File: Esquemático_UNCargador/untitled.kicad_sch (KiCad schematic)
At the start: 18 parts, among them U3.3 LM2596S-3.3, U5 LM2596S-5

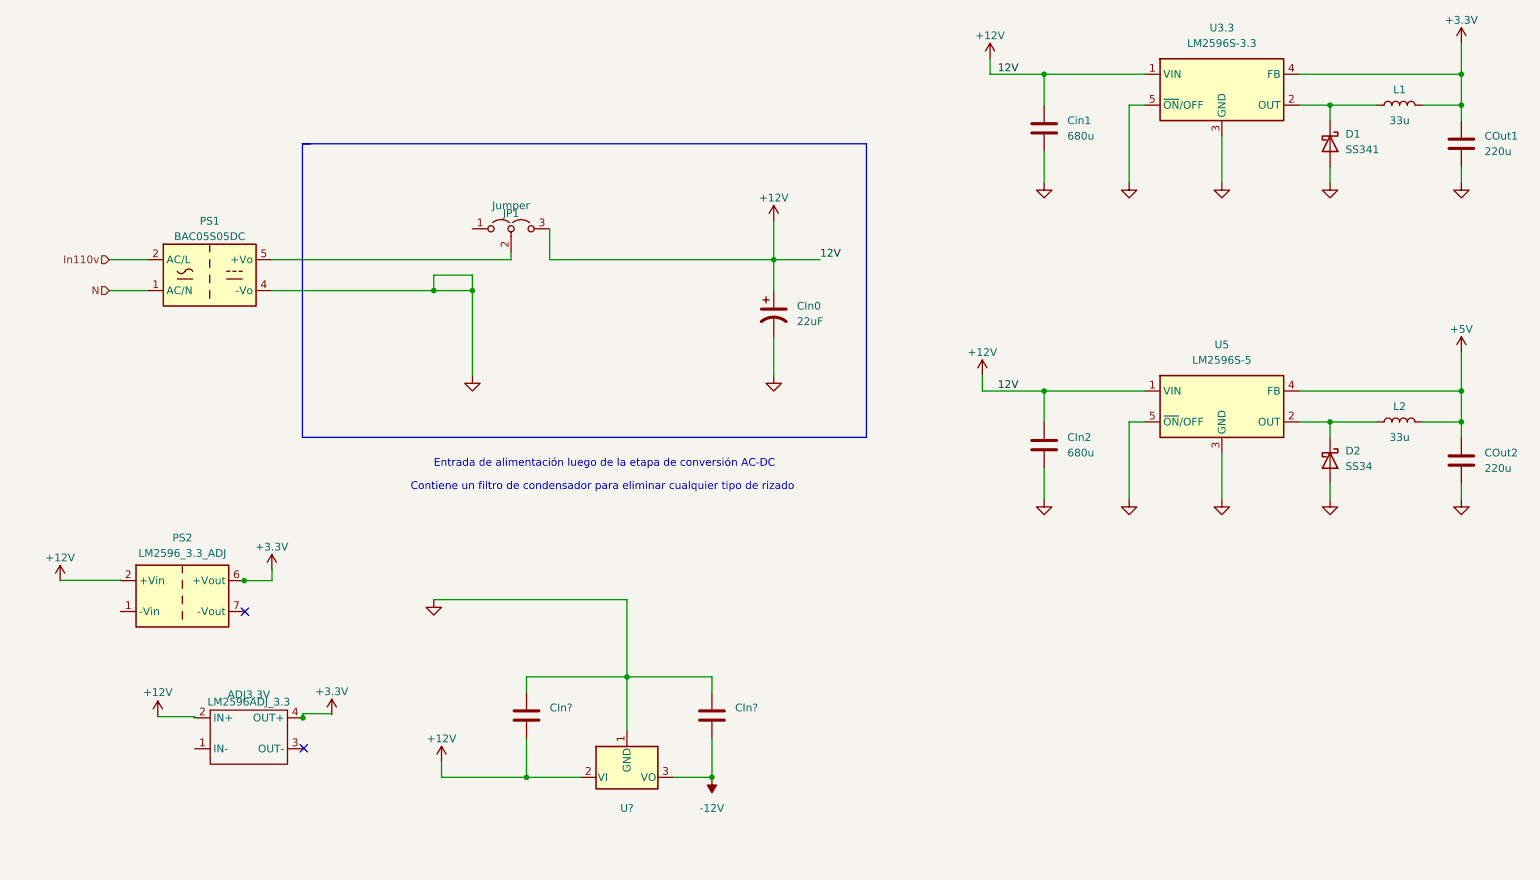
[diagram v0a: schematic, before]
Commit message: CorrecciónPotencia
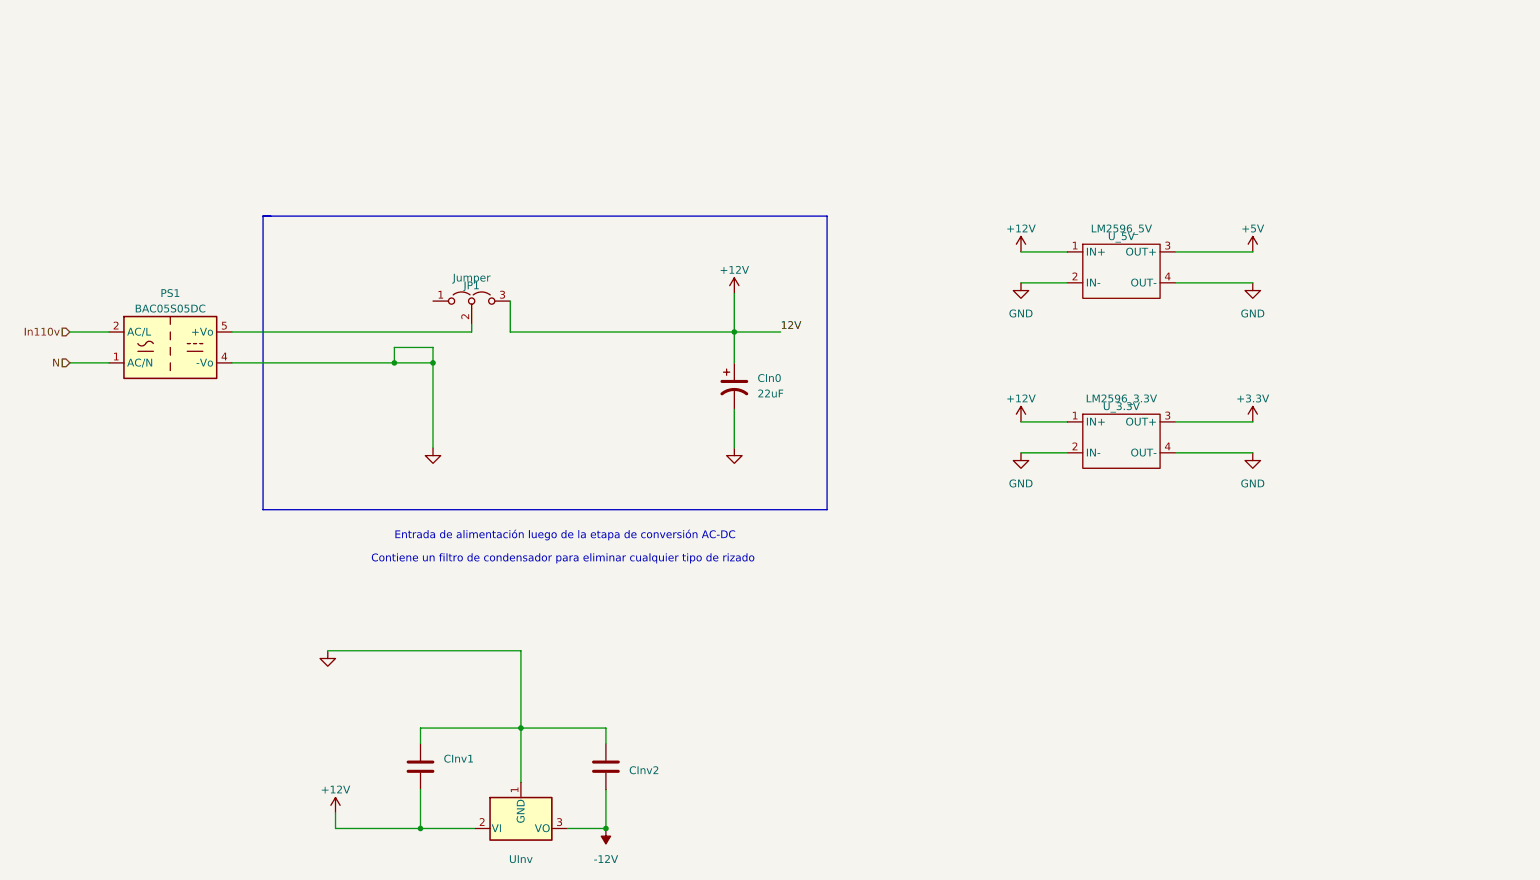
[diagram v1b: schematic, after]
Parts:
- removed CIn2, Cin1: 680u, Capacitor_THT:C_Radial_D10.0mm_H16.0mm_P5.00mm, symbol Device:C
- removed COut1, COut2: 220u, Capacitor_SMD:CP_Elec_8x10, symbol Device:C
- removed D1: SS341, Diode_SMD:D_SMA_Handsoldering, symbol Diode:1N5822
- removed D2: SS34, Diode_SMD:D_SMA_Handsoldering, symbol Diode:1N5822
- removed L1, L2: 33u, Inductor_SMD:L_12x12mm_H8mm, symbol Device:L
- removed LM2596ADJ_3.3: ADJ3.3V, LM2596ADJ:LM2596ADJ, symbol LM2596ADJ:LM2596ADJ
- removed PS2: LM2596_3.3_ADJ, LM2596ADJ:LM2596ADJ, symbol Converter_DCDC:ITX0503SA-H
- removed U3.3: LM2596S-3.3, Package_TO_SOT_SMD:TO-263-5_TabPin3, symbol Regulator_Switching:LM2596S-3.3
- removed U5: LM2596S-5, Package_TO_SOT_THT:TO-220-5_Vertical, symbol Regulator_Switching:LM2596S-5
- added U_3.3V: LM2596_3.3V, LM2596ADJ:LM2596ADJ, symbol LM2596ADJ:LM2596ADJ
- added U_5V: LM2596_5V, LM2596ADJ:LM2596ADJ, symbol LM2596ADJ:LM2596ADJ
- gave numbers to parts that had none: 3
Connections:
- net +12V: now also U_3.3V.1 (IN+), U_5V.1 (IN+)
- net +3.3V: now also U_3.3V.3 (OUT+)
- net +5V: now also U_5V.3 (OUT+)
- net GND: now also U_3.3V.2 (IN-), U_3.3V.4 (OUT-), U_5V.2 (IN-), U_5V.4 (OUT-)
- no-connect marks 2 -> 0
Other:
- moved on the sheet: CIn0, CInv1, CInv2, JP1, PS1, UInv
